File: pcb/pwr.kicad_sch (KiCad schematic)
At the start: 7 parts, among them U2 MCP73831-2-OT

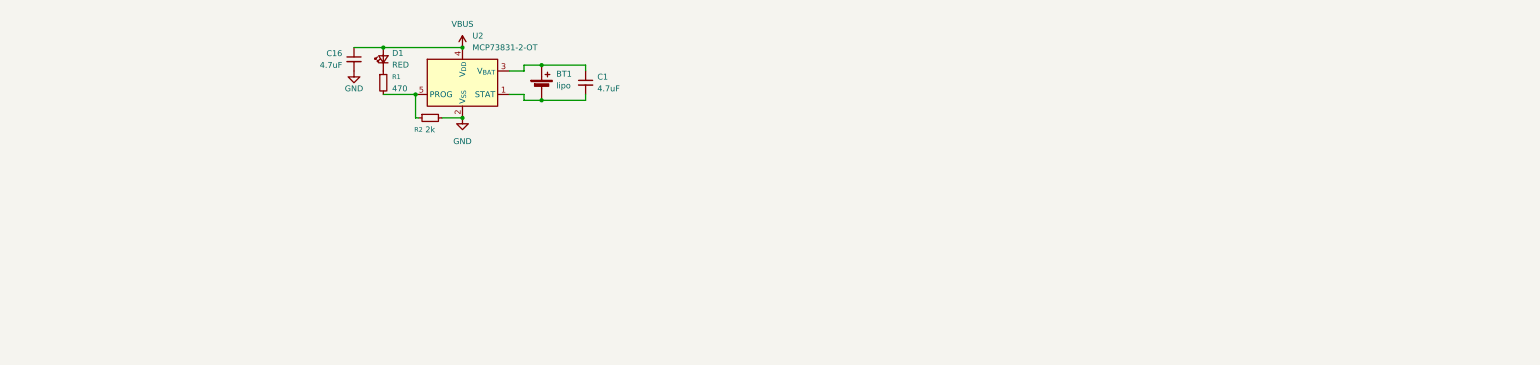
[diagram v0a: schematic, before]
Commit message: sussy
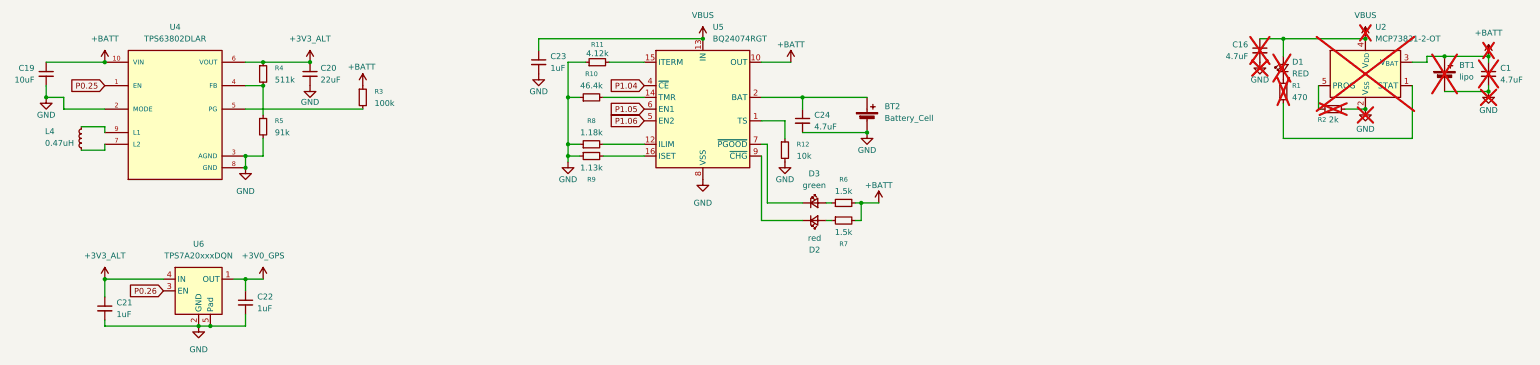
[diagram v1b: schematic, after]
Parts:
- added BT2: Battery_Cell, symbol Device:Battery_Cell
- added C19: 10uF, symbol Device:C_Small
- added C20: 22uF, symbol Device:C_Small
- added C21, C22, C23: 1uF, symbol Device:C_Small
- added C24: 4.7uF, symbol Device:C_Small
- added D2: red, symbol Device:LED_Small
- added D3: green, symbol Device:LED_Small
- added L4: 0.47uH, symbol Device:L_Small
- added R10: 46.4k, symbol Device:R_Small
- added R11: 4.12k, symbol Device:R_Small
- added R12: 10k, symbol Device:R_Small
- added R3: 100k, symbol Device:R_Small
- added R4: 511k, symbol Device:R_Small
- added R5: 91k, symbol Device:R_Small
- added R6, R7: 1.5k, symbol Device:R_Small
- added R8: 1.18k, symbol Device:R_Small
- added R9: 1.13k, symbol Device:R_Small
- added U4: TPS63802DLAR, TPS63802DLAR:VREG_TPS63802DLAR, symbol TPS63802:TPS63802DLAR
- added U5: BQ24074RGT, Package_DFN_QFN:VQFN-16-1EP_3x3mm_P0.5mm_EP1.6x1.6mm, symbol Battery_Management:BQ24074RGT
- added U6: TPS7A20xxxDQN, Package_SON:Texas_X2SON-4_1x1mm_P0.65mm, symbol Regulator_Linear:TPS7A20xxxDQN
- BT1, C1, C16, D1, R1, R2, U2: now not fitted; now left out of the parts list
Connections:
- net GND: now also BT1.2 (-), C1.2, BT2.2 (-), C19.2, C20.2, C21.2, C22.2, C23.2, C24.2, R10.1, R11.1, R12.2, R5.2, R8.1, R9.1, U4.2 (MODE), U4.3 (AGND), U4.8 (GND), U5.17 (VSS), U5.8 (VSS), U6.2 (GND), U6.5 (Pad)
- net VBUS: now also C23.1, U5.13 (IN)
- net at R2.1, U2.5 (PROG): no longer R1.2
- net +BATT: now reaches BT1.1 (+), C1.1, U2.3 (V_{BAT})
- net +BATT: now also C19.1, R3.1, R6.2, R7.2, U4.10 (VIN), U5.10 (OUT), U5.11 (OUT)
- new net: D3.1 (K), U5.7 (~{PGOOD})
- new net: D3.2 (A), R6.1
- new net: R12.1, U5.1 (TS)
- new net: R10.2, U5.14 (TMR)
- new net: R4.2, R5.1, U4.4 (FB)
- new net: R3.2, U4.5 (PG)
- new net: L4.1, U4.7 (L2)
- new net: L4.2, U4.9 (L1)
- new net: D2.1 (K), U5.9 (~{CHG})
- new net: D2.2 (A), R7.1
- new net: R1.2, U2.1 (STAT)
- new net: R8.2, U5.12 (ILIM)
- new net: R11.2, U5.15 (ITERM)
- new net: R9.2, U5.16 (ISET)
- new net: BT2.1 (+), C24.1, U5.2 (BAT), U5.3 (BAT)
- new net +3V0_GPS: C22.1, U6.1 (OUT)
- new net +3V3_ALT: C20.1, C21.1, R4.1, U4.6 (VOUT), U6.4 (IN)
- new net P0.25: U4.1 (EN)
- new net P0.26: U6.3 (EN)
- new net P1.04: U5.4 (~{CE})
- new net P1.05: U5.6 (EN1)
- new net P1.06: U5.5 (EN2)
